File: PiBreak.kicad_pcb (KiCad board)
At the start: 2 copper layers, 56 x 62.9 mm, 318 parts, among them P1 RASPBERRY_PI_P1, P2 CONN_17, P3 CONN_8, P4 CONN_8, P5 CONN_8, P6 CONN_4X2

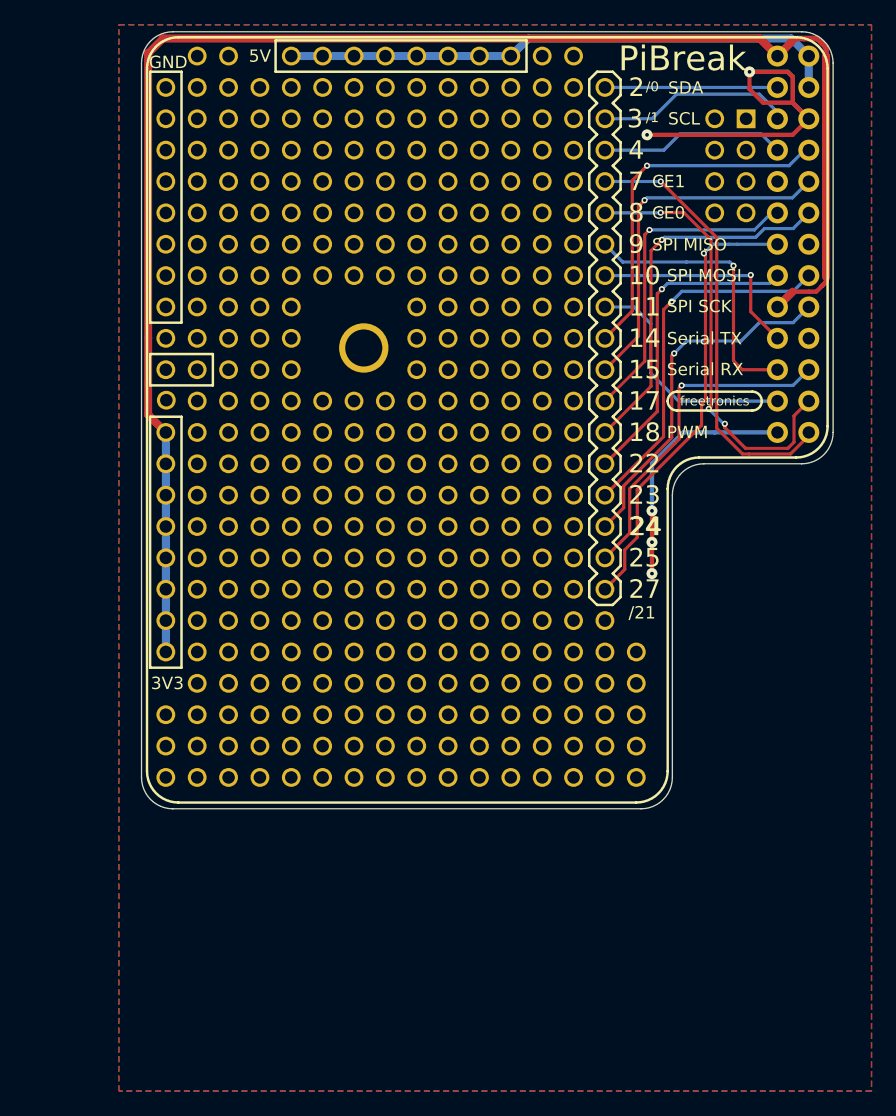
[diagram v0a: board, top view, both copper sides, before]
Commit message: Bump version to 1.0
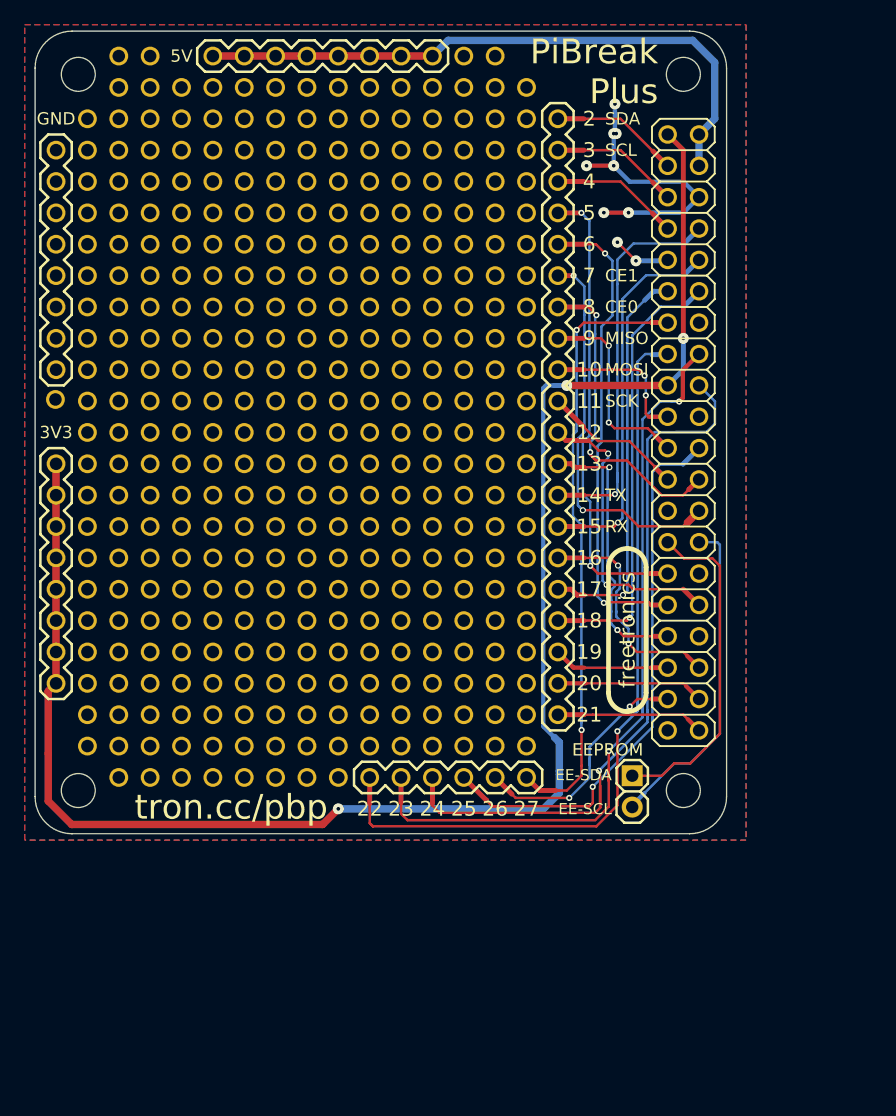
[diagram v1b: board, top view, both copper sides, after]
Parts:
- removed the 1pin_prototyping at (214.7, 124.4)
- removed the 1pin_prototyping at (224.8, 154.9)
- removed the 1pin_prototyping at (245.1, 147.3)
- removed the 1pin_prototyping at (247.7, 147.3)
- removed the 1pin_prototyping at (247.7, 142.2)
- removed the 1pin_prototyping at (245.1, 142.2)
- removed the 1pin_prototyping at (242.6, 142.2)
- removed the 1pin_prototyping at (240.0, 142.2)
- removed the 1pin_prototyping at (240.0, 144.8)
- removed the 1pin_prototyping at (242.6, 144.8)
- removed the 1pin_prototyping at (245.1, 144.8)
- removed the 1pin_prototyping at (247.7, 144.8)
- removed the 1pin_prototyping at (227.3, 154.9)
- removed the 1pin_prototyping at (227.3, 149.9)
- removed the 1pin_prototyping at (224.8, 149.9)
- removed the 1pin_prototyping at (222.2, 149.9)
- removed the 1pin_prototyping at (219.7, 149.9)
- removed the 1pin_prototyping at (219.7, 147.3)
- removed the 1pin_prototyping at (222.2, 147.3)
- removed the 1pin_prototyping at (224.8, 147.3)
- removed the 1pin_prototyping at (227.3, 147.3)
- removed the 1pin_prototyping at (227.3, 142.2)
- removed the 1pin_prototyping at (224.8, 142.2)
- removed the 1pin_prototyping at (247.7, 152.4)
- removed the 1pin_prototyping at (222.2, 142.2)
- removed the 1pin_prototyping at (219.7, 142.2)
- removed the 1pin_prototyping at (219.7, 144.8)
- removed the 1pin_prototyping at (222.2, 144.8)
- removed the 1pin_prototyping at (224.8, 144.8)
- removed the 1pin_prototyping at (227.3, 144.8)
- removed the 1pin_prototyping at (227.3, 137.2)
- removed the 1pin_prototyping at (224.8, 137.2)
- removed the 1pin_prototyping at (222.2, 137.2)
- removed the 1pin_prototyping at (219.7, 137.2)
- removed the 1pin_prototyping at (245.1, 152.4)
- removed the 1pin_prototyping at (219.7, 139.7)
- removed the 1pin_prototyping at (222.2, 139.7)
- removed the 1pin_prototyping at (224.8, 139.7)
- removed the 1pin_prototyping at (227.3, 139.7)
- removed the 1pin_prototyping at (247.7, 137.2)
- removed the 1pin_prototyping at (245.1, 137.2)
- removed the 1pin_prototyping at (242.6, 137.2)
- removed the 1pin_prototyping at (240.0, 137.2)
- removed the 1pin_prototyping at (240.0, 139.7)
- removed the 1pin_prototyping at (242.6, 139.7)
- removed the 1pin_prototyping at (242.6, 152.4)
- removed the 1pin_prototyping at (245.1, 139.7)
- removed the 1pin_prototyping at (247.7, 139.7)
- removed the 1pin_prototyping at (237.5, 139.7)
- removed the 1pin_prototyping at (234.9, 139.7)
- removed the 1pin_prototyping at (232.4, 139.7)
- removed the 1pin_prototyping at (229.9, 139.7)
- removed the 1pin_prototyping at (229.9, 137.2)
- removed the 1pin_prototyping at (232.4, 137.2)
- removed the 1pin_prototyping at (234.9, 137.2)
- removed the 1pin_prototyping at (237.5, 137.2)
- removed the 1pin_prototyping at (240.0, 152.4)
- removed the 1pin_prototyping at (237.5, 119.4)
- removed the 1pin_prototyping at (234.9, 119.4)
- removed the 1pin_prototyping at (234.9, 121.9)
- removed the 1pin_prototyping at (237.5, 121.9)
- removed the 1pin_prototyping at (247.7, 121.9)
- removed the 1pin_prototyping at (245.1, 121.9)
- removed the 1pin_prototyping at (242.6, 121.9)
- removed the 1pin_prototyping at (240.0, 121.9)
- removed the 1pin_prototyping at (240.0, 119.4)
- removed the 1pin_prototyping at (242.6, 119.4)
- removed the 1pin_prototyping at (240.0, 154.9)
- removed the 1pin_prototyping at (245.1, 119.4)
- removed the 1pin_prototyping at (247.7, 119.4)
- removed the 1pin_prototyping at (224.8, 121.9)
- removed the 1pin_prototyping at (222.2, 121.9)
- removed the 1pin_prototyping at (219.7, 121.9)
- removed the 1pin_prototyping at (219.7, 119.4)
- removed the 1pin_prototyping at (222.2, 119.4)
- removed the 1pin_prototyping at (224.8, 119.4)
- removed the 1pin_prototyping at (227.3, 127.0)
- removed the 1pin_prototyping at (224.8, 127.0)
- removed the 1pin_prototyping at (242.6, 154.9)
- removed the 1pin_prototyping at (222.2, 127.0)
- removed the 1pin_prototyping at (219.7, 127.0)
- removed the 1pin_prototyping at (219.7, 124.5)
- removed the 1pin_prototyping at (222.2, 124.5)
- removed the 1pin_prototyping at (224.8, 124.5)
- removed the 1pin_prototyping at (227.3, 124.5)
- removed the 1pin_prototyping at (227.3, 129.5)
- removed the 1pin_prototyping at (224.8, 129.5)
- removed the 1pin_prototyping at (222.2, 129.5)
- removed the 1pin_prototyping at (219.7, 129.5)
- removed the 1pin_prototyping at (245.1, 154.9)
- removed the 1pin_prototyping at (219.7, 132.1)
- removed the 1pin_prototyping at (222.2, 132.1)
- removed the 1pin_prototyping at (224.8, 132.1)
- removed the 1pin_prototyping at (227.3, 132.1)
- removed the 1pin_prototyping at (247.7, 127.0)
- removed the 1pin_prototyping at (245.1, 127.0)
- removed the 1pin_prototyping at (242.6, 127.0)
- removed the 1pin_prototyping at (240.0, 127.0)
- removed the 1pin_prototyping at (240.0, 124.5)
- removed the 1pin_prototyping at (242.6, 124.5)
- removed the 1pin_prototyping at (247.7, 154.9)
- removed the 1pin_prototyping at (245.1, 124.5)
- removed the 1pin_prototyping at (247.7, 124.5)
- removed the 1pin_prototyping at (247.7, 129.5)
- removed the 1pin_prototyping at (245.1, 129.5)
- removed the 1pin_prototyping at (242.6, 129.5)
- removed the 1pin_prototyping at (240.0, 129.5)
- removed the 1pin_prototyping at (240.0, 132.1)
- removed the 1pin_prototyping at (242.6, 132.1)
- removed the 1pin_prototyping at (245.1, 132.1)
- removed the 1pin_prototyping at (247.7, 132.1)
- removed the 1pin_prototyping at (214.6, 119.4)
- removed the 1pin_prototyping at (237.5, 154.9)
- removed the 1pin_prototyping at (237.5, 132.1)
- removed the 1pin_prototyping at (234.9, 132.1)
- removed the 1pin_prototyping at (232.4, 132.1)
- removed the 1pin_prototyping at (229.9, 132.1)
- removed the 1pin_prototyping at (229.9, 129.5)
- removed the 1pin_prototyping at (232.4, 129.5)
- removed the 1pin_prototyping at (234.9, 129.5)
- removed the 1pin_prototyping at (237.5, 129.5)
- removed the 1pin_prototyping at (237.5, 124.5)
- removed the 1pin_prototyping at (234.9, 124.5)
- removed the 1pin_prototyping at (234.9, 154.9)
- removed the 1pin_prototyping at (232.4, 124.5)
- removed the 1pin_prototyping at (229.9, 124.5)
- removed the 1pin_prototyping at (229.9, 127.0)
- removed the 1pin_prototyping at (232.4, 127.0)
- removed the 1pin_prototyping at (234.9, 127.0)
- removed the 1pin_prototyping at (237.5, 127.0)
- removed the 1pin_prototyping at (237.5, 111.8)
- removed the 1pin_prototyping at (234.9, 111.8)
- removed the 1pin_prototyping at (232.4, 111.8)
- removed the 1pin_prototyping at (229.9, 111.8)
- removed the 1pin_prototyping at (232.4, 154.9)
- removed the 1pin_prototyping at (229.9, 109.2)
- removed the 1pin_prototyping at (232.4, 109.2)
- removed the 1pin_prototyping at (234.9, 109.2)
- removed the 1pin_prototyping at (237.5, 109.2)
- removed the 1pin_prototyping at (237.5, 114.3)
- removed the 1pin_prototyping at (234.9, 114.3)
- removed the 1pin_prototyping at (232.4, 114.3)
- removed the 1pin_prototyping at (229.9, 114.3)
- removed the 1pin_prototyping at (234.9, 116.8)
- removed the 1pin_prototyping at (237.5, 116.8)
- removed the 1pin_prototyping at (229.9, 154.9)
- removed the 1pin_prototyping at (247.7, 116.8)
- removed the 1pin_prototyping at (245.1, 116.8)
- removed the 1pin_prototyping at (242.6, 116.8)
- removed the 1pin_prototyping at (240.0, 116.8)
- removed the 1pin_prototyping at (240.0, 114.3)
- removed the 1pin_prototyping at (242.6, 114.3)
- removed the 1pin_prototyping at (245.1, 114.3)
- removed the 1pin_prototyping at (247.7, 114.3)
- removed the 1pin_prototyping at (247.7, 109.2)
- removed the 1pin_prototyping at (245.1, 109.2)
- removed the 1pin_prototyping at (229.9, 152.4)
- removed the 1pin_prototyping at (242.6, 109.2)
- removed the 1pin_prototyping at (240.0, 109.2)
- removed the 1pin_prototyping at (240.0, 111.8)
- removed the 1pin_prototyping at (242.6, 111.8)
- removed the 1pin_prototyping at (245.1, 111.8)
- removed the 1pin_prototyping at (247.7, 111.8)
- removed the 1pin_prototyping at (224.8, 116.8)
- removed the 1pin_prototyping at (222.2, 116.8)
- removed the 1pin_prototyping at (219.7, 116.8)
- removed the 1pin_prototyping at (219.7, 114.3)
- removed the 1pin_prototyping at (232.4, 152.4)
- removed the 1pin_prototyping at (222.2, 114.3)
- removed the 1pin_prototyping at (224.8, 114.3)
- removed the 1pin_prototyping at (227.3, 114.3)
- removed the 1pin_prototyping at (227.3, 109.2)
- removed the 1pin_prototyping at (224.8, 109.2)
- removed the 1pin_prototyping at (222.2, 109.2)
- removed the 1pin_prototyping at (219.7, 109.2)
- removed the 1pin_prototyping at (219.7, 111.8)
- removed the 1pin_prototyping at (222.2, 111.8)
- removed the 1pin_prototyping at (224.8, 111.8)
- removed the 1pin_prototyping at (234.9, 152.4)
- removed the 1pin_prototyping at (227.3, 111.8)
- removed the 1pin_prototyping at (219.7, 96.5)
- removed the 1pin_prototyping at (227.3, 101.6)
- removed the 1pin_prototyping at (224.8, 101.6)
- removed the 1pin_prototyping at (222.2, 101.6)
- removed the 1pin_prototyping at (219.7, 101.6)
- removed the 1pin_prototyping at (219.7, 99.1)
- removed the 1pin_prototyping at (222.2, 99.1)
- removed the 1pin_prototyping at (224.8, 99.1)
- removed the 1pin_prototyping at (227.3, 99.1)
- removed the 1pin_prototyping at (237.5, 152.4)
- removed the 1pin_prototyping at (227.3, 104.1)
- removed the 1pin_prototyping at (224.8, 104.1)
- removed the 1pin_prototyping at (222.2, 104.1)
- removed the 1pin_prototyping at (219.7, 104.1)
- removed the 1pin_prototyping at (219.7, 106.7)
- removed the 1pin_prototyping at (222.2, 106.7)
- removed the 1pin_prototyping at (224.8, 106.7)
- removed the 1pin_prototyping at (227.3, 106.7)
- removed the 1pin_prototyping at (247.7, 96.5)
- removed the 1pin_prototyping at (245.1, 96.5)
- removed the 1pin_prototyping at (252.7, 154.9)
- removed the 1pin_prototyping at (247.7, 101.6)
- removed the 1pin_prototyping at (245.1, 101.6)
- removed the 1pin_prototyping at (242.6, 101.6)
- removed the 1pin_prototyping at (240.0, 101.6)
- removed the 1pin_prototyping at (240.0, 99.1)
- removed the 1pin_prototyping at (242.6, 99.1)
- removed the 1pin_prototyping at (245.1, 99.1)
- removed the 1pin_prototyping at (247.7, 99.1)
- removed the 1pin_prototyping at (247.7, 104.1)
- removed the 1pin_prototyping at (245.1, 104.1)
- removed the 1pin_prototyping at (250.2, 154.9)
- removed the 1pin_prototyping at (242.6, 104.1)
- removed the 1pin_prototyping at (240.0, 104.1)
- removed the 1pin_prototyping at (240.0, 106.7)
- removed the 1pin_prototyping at (242.6, 106.7)
- removed the 1pin_prototyping at (245.1, 106.7)
- removed the 1pin_prototyping at (247.7, 106.7)
- removed the 1pin_prototyping at (237.5, 106.7)
- removed the 1pin_prototyping at (234.9, 106.7)
- removed the 1pin_prototyping at (232.4, 106.7)
- removed the 1pin_prototyping at (229.9, 106.7)
- removed the 1pin_prototyping at (217.2, 121.9)
- removed the 1pin_prototyping at (250.2, 152.4)
- removed the 1pin_prototyping at (229.9, 104.1)
- removed the 1pin_prototyping at (232.4, 104.1)
- removed the 1pin_prototyping at (234.9, 104.1)
- removed the 1pin_prototyping at (237.5, 104.1)
- removed the 1pin_prototyping at (237.5, 99.1)
- removed the 1pin_prototyping at (234.9, 99.1)
- removed the 1pin_prototyping at (232.4, 99.1)
- removed the 1pin_prototyping at (229.9, 99.1)
- removed the 1pin_prototyping at (229.9, 101.6)
- removed the 1pin_prototyping at (232.4, 101.6)
- removed the 1pin_prototyping at (252.7, 152.4)
- removed the 1pin_prototyping at (234.9, 101.6)
- removed the 1pin_prototyping at (237.5, 101.6)
- removed the 1pin_prototyping at (217.2, 154.9)
- removed the 1pin_prototyping at (214.6, 154.9)
- removed the 1pin_prototyping at (214.6, 152.4)
- removed the 1pin_prototyping at (217.2, 152.4)
- removed the 1pin_prototyping at (217.2, 106.7)
- removed the 1pin_prototyping at (217.2, 104.1)
- removed the 1pin_prototyping at (217.2, 99.1)
- removed the 1pin_prototyping at (217.2, 101.6)
- removed the 1pin_prototyping at (227.3, 152.4)
- removed the 1pin_prototyping at (217.2, 96.5)
- removed the 1pin_prototyping at (217.2, 111.8)
- removed the 1pin_prototyping at (217.2, 109.2)
- removed the 1pin_prototyping at (217.2, 114.3)
- removed the 1pin_prototyping at (217.2, 116.8)
- removed the 1pin_prototyping at (217.2, 132.1)
- removed the 1pin_prototyping at (217.2, 129.5)
- removed the 1pin_prototyping at (217.2, 124.5)
- removed the 1pin_prototyping at (217.2, 127.0)
- removed the 1pin_prototyping at (217.2, 119.4)
- removed the 1pin_prototyping at (224.8, 152.4)
- removed the 1pin_prototyping at (214.6, 121.9)
- removed the 1pin_prototyping at (217.2, 139.7)
- removed the 1pin_prototyping at (217.2, 137.2)
- removed the 1pin_prototyping at (217.2, 134.6)
- removed the 1pin_prototyping at (217.2, 144.8)
- removed the 1pin_prototyping at (217.2, 142.2)
- removed the 1pin_prototyping at (217.2, 147.3)
- removed the 1pin_prototyping at (214.6, 149.9)
- removed the 1pin_prototyping at (217.2, 149.9)
- removed the 1pin_prototyping at (252.7, 144.8)
- removed the 1pin_prototyping at (222.2, 152.4)
- removed the 1pin_prototyping at (250.2, 144.8)
- removed the 1pin_prototyping at (250.2, 142.2)
- removed the 1pin_prototyping at (252.7, 147.3)
- removed the 1pin_prototyping at (250.2, 147.3)
- removed the 1pin_prototyping at (250.2, 149.9)
- removed the 1pin_prototyping at (252.7, 149.9)
- removed the 1pin_prototyping at (219.7, 134.6)
- removed the 1pin_prototyping at (222.2, 134.6)
- removed the 1pin_prototyping at (224.8, 134.6)
- removed the 1pin_prototyping at (227.3, 134.6)
- removed the 1pin_prototyping at (219.7, 152.4)
- removed the 1pin_prototyping at (240.0, 134.6)
- removed the 1pin_prototyping at (242.6, 134.6)
- removed the 1pin_prototyping at (245.1, 134.6)
- removed the 1pin_prototyping at (247.7, 134.6)
- removed the 1pin_prototyping at (237.5, 134.6)
- removed the 1pin_prototyping at (234.9, 134.6)
- removed the 1pin_prototyping at (232.4, 134.6)
- removed the 1pin_prototyping at (229.9, 134.6)
- removed the 1pin_prototyping at (237.5, 144.8)
- removed the 1pin_prototyping at (234.9, 144.8)
- removed the 1pin_prototyping at (219.7, 154.9)
- removed the 1pin_prototyping at (232.4, 144.8)
- removed the 1pin_prototyping at (229.9, 144.8)
- removed the 1pin_prototyping at (229.9, 142.2)
- removed the 1pin_prototyping at (232.4, 142.2)
- removed the 1pin_prototyping at (234.9, 142.2)
- removed the 1pin_prototyping at (237.5, 142.2)
- removed the 1pin_prototyping at (237.5, 147.3)
- removed the 1pin_prototyping at (234.9, 147.3)
- removed the 1pin_prototyping at (232.4, 147.3)
- removed the 1pin_prototyping at (229.9, 147.3)
- removed the 1pin_prototyping at (222.2, 154.9)
- removed the 1pin_prototyping at (229.9, 149.9)
- removed the 1pin_prototyping at (232.4, 149.9)
- removed the 1pin_prototyping at (234.9, 149.9)
- removed the 1pin_prototyping at (237.5, 149.9)
- removed the 1pin_prototyping at (247.7, 149.9)
- removed the 1pin_prototyping at (245.1, 149.9)
- removed the 1pin_prototyping at (242.6, 149.9)
- removed the 1pin_prototyping at (240.0, 149.9)
- removed the 1pin_prototyping at (240.0, 147.3)
- removed the 1pin_prototyping at (242.6, 147.3)
- removed LOGO_FREETRONICS_SMALL: val**, LOGO_FREETRONICS_SMALL
- added 1PIN: P***, Connect:1pin, F.Cu at (256.8, 99.0)
- added 1PIN: P***, Connect:1pin, F.Cu at (248.8, 98.0)
- added 1PIN: P***, Connect:1pin, F.Cu at (250.2, 156.2)
- added 1PIN: P***, Connect:1pin, F.Cu at (256.8, 157.0)
- added 1pin_prototyping: val**, FT:1pin_prototyping, F.Cu at (210.8, 96.5)
- added 1pin_prototyping: val**, FT:1pin_prototyping, F.Cu at (208.3, 106.7)
- added 1pin_prototyping: val**, FT:1pin_prototyping, F.Cu at (210.8, 106.7)
- added 1pin_prototyping: val**, FT:1pin_prototyping, F.Cu at (210.8, 101.6)
- added 1pin_prototyping: val**, FT:1pin_prototyping, F.Cu at (213.4, 101.6)
- added 1pin_prototyping: val**, FT:1pin_prototyping, F.Cu at (213.4, 104.1)
- added 1pin_prototyping: val**, FT:1pin_prototyping, F.Cu at (210.8, 104.1)
- added 1pin_prototyping: val**, FT:1pin_prototyping, F.Cu at (213.4, 111.8)
- added 1pin_prototyping: val**, FT:1pin_prototyping, F.Cu at (210.8, 111.8)
- added 1pin_prototyping: val**, FT:1pin_prototyping, F.Cu at (215.9, 111.8)
- added 1pin_prototyping: val**, FT:1pin_prototyping, F.Cu at (218.4, 111.8)
- added 1pin_prototyping: val**, FT:1pin_prototyping, F.Cu at (221.0, 111.8)
- added 1pin_prototyping: val**, FT:1pin_prototyping, F.Cu at (208.3, 109.2)
- added 1pin_prototyping: val**, FT:1pin_prototyping, F.Cu at (223.5, 111.8)
- added 1pin_prototyping: val**, FT:1pin_prototyping, F.Cu at (226.1, 111.8)
- added 1pin_prototyping: val**, FT:1pin_prototyping, F.Cu at (228.6, 111.8)
- added 1pin_prototyping: val**, FT:1pin_prototyping, F.Cu at (243.8, 111.8)
- added 1pin_prototyping: val**, FT:1pin_prototyping, F.Cu at (241.3, 111.8)
- added 1pin_prototyping: val**, FT:1pin_prototyping, F.Cu at (238.8, 111.8)
- added 1pin_prototyping: val**, FT:1pin_prototyping, F.Cu at (236.2, 111.8)
- added 1pin_prototyping: val**, FT:1pin_prototyping, F.Cu at (233.7, 111.8)
- added 1pin_prototyping: val**, FT:1pin_prototyping, F.Cu at (231.1, 111.8)
- added 1pin_prototyping: val**, FT:1pin_prototyping, F.Cu at (231.1, 132.1)
- added 1pin_prototyping: val**, FT:1pin_prototyping, F.Cu at (208.3, 124.5)
- added 1pin_prototyping: val**, FT:1pin_prototyping, F.Cu at (233.7, 132.1)
- added 1pin_prototyping: val**, FT:1pin_prototyping, F.Cu at (236.2, 132.1)
- added 1pin_prototyping: val**, FT:1pin_prototyping, F.Cu at (238.8, 132.1)
- added 1pin_prototyping: val**, FT:1pin_prototyping, F.Cu at (241.3, 132.1)
- added 1pin_prototyping: val**, FT:1pin_prototyping, F.Cu at (241.3, 129.5)
- added 1pin_prototyping: val**, FT:1pin_prototyping, F.Cu at (238.8, 129.5)
- added 1pin_prototyping: val**, FT:1pin_prototyping, F.Cu at (236.2, 129.5)
- added 1pin_prototyping: val**, FT:1pin_prototyping, F.Cu at (233.7, 129.5)
- added 1pin_prototyping: val**, FT:1pin_prototyping, F.Cu at (231.1, 129.5)
- added 1pin_prototyping: val**, FT:1pin_prototyping, F.Cu at (231.1, 124.5)
- added 1pin_prototyping: val**, FT:1pin_prototyping, F.Cu at (205.7, 124.3)
- added 1pin_prototyping: val**, FT:1pin_prototyping, F.Cu at (233.7, 124.5)
- added 1pin_prototyping: val**, FT:1pin_prototyping, F.Cu at (236.2, 124.5)
- added 1pin_prototyping: val**, FT:1pin_prototyping, F.Cu at (238.8, 124.5)
- added 1pin_prototyping: val**, FT:1pin_prototyping, F.Cu at (241.3, 124.5)
- added 1pin_prototyping: val**, FT:1pin_prototyping, F.Cu at (241.3, 127.0)
- added 1pin_prototyping: val**, FT:1pin_prototyping, F.Cu at (238.8, 127.0)
- added 1pin_prototyping: val**, FT:1pin_prototyping, F.Cu at (236.2, 127.0)
- added 1pin_prototyping: val**, FT:1pin_prototyping, F.Cu at (233.7, 127.0)
- added 1pin_prototyping: val**, FT:1pin_prototyping, F.Cu at (231.1, 127.0)
- added 1pin_prototyping: val**, FT:1pin_prototyping, F.Cu at (243.8, 127.0)
- added 1pin_prototyping: val**, FT:1pin_prototyping, F.Cu at (228.6, 154.9)
- added 1pin_prototyping: val**, FT:1pin_prototyping, F.Cu at (243.8, 124.5)
- added 1pin_prototyping: val**, FT:1pin_prototyping, F.Cu at (243.8, 129.5)
- added 1pin_prototyping: val**, FT:1pin_prototyping, F.Cu at (243.8, 132.1)
- added 1pin_prototyping: val**, FT:1pin_prototyping, F.Cu at (228.6, 132.1)
- added 1pin_prototyping: val**, FT:1pin_prototyping, F.Cu at (228.6, 129.5)
- added 1pin_prototyping: val**, FT:1pin_prototyping, F.Cu at (228.6, 124.5)
- added 1pin_prototyping: val**, FT:1pin_prototyping, F.Cu at (228.6, 127.0)
- added 1pin_prototyping: val**, FT:1pin_prototyping, F.Cu at (215.9, 127.0)
- added 1pin_prototyping: val**, FT:1pin_prototyping, F.Cu at (218.4, 127.0)
- added 1pin_prototyping: val**, FT:1pin_prototyping, F.Cu at (221.0, 127.0)
- added 1pin_prototyping: val**, FT:1pin_prototyping, F.Cu at (226.1, 154.9)
- added 1pin_prototyping: val**, FT:1pin_prototyping, F.Cu at (223.5, 127.0)
- added 1pin_prototyping: val**, FT:1pin_prototyping, F.Cu at (226.1, 127.0)
- added 1pin_prototyping: val**, FT:1pin_prototyping, F.Cu at (226.1, 124.5)
- added 1pin_prototyping: val**, FT:1pin_prototyping, F.Cu at (223.5, 124.5)
- added 1pin_prototyping: val**, FT:1pin_prototyping, F.Cu at (221.0, 124.5)
- added 1pin_prototyping: val**, FT:1pin_prototyping, F.Cu at (218.4, 124.5)
- added 1pin_prototyping: val**, FT:1pin_prototyping, F.Cu at (215.9, 124.5)
- added 1pin_prototyping: val**, FT:1pin_prototyping, F.Cu at (215.9, 129.5)
- added 1pin_prototyping: val**, FT:1pin_prototyping, F.Cu at (218.4, 129.5)
- added 1pin_prototyping: val**, FT:1pin_prototyping, F.Cu at (221.0, 129.5)
- added 1pin_prototyping: val**, FT:1pin_prototyping, F.Cu at (223.5, 154.9)
- added 1pin_prototyping: val**, FT:1pin_prototyping, F.Cu at (223.5, 129.5)
- added 1pin_prototyping: val**, FT:1pin_prototyping, F.Cu at (226.1, 129.5)
- added 1pin_prototyping: val**, FT:1pin_prototyping, F.Cu at (226.1, 132.1)
- added 1pin_prototyping: val**, FT:1pin_prototyping, F.Cu at (223.5, 132.1)
- added 1pin_prototyping: val**, FT:1pin_prototyping, F.Cu at (221.0, 132.1)
- added 1pin_prototyping: val**, FT:1pin_prototyping, F.Cu at (218.4, 132.1)
- added 1pin_prototyping: val**, FT:1pin_prototyping, F.Cu at (215.9, 132.1)
- added 1pin_prototyping: val**, FT:1pin_prototyping, F.Cu at (210.8, 132.1)
- added 1pin_prototyping: val**, FT:1pin_prototyping, F.Cu at (213.4, 132.1)
- added 1pin_prototyping: val**, FT:1pin_prototyping, F.Cu at (213.4, 129.5)
- added 1pin_prototyping: val**, FT:1pin_prototyping, F.Cu at (221.0, 154.9)
- added 1pin_prototyping: val**, FT:1pin_prototyping, F.Cu at (210.8, 129.5)
- added 1pin_prototyping: val**, FT:1pin_prototyping, F.Cu at (210.8, 124.5)
- added 1pin_prototyping: val**, FT:1pin_prototyping, F.Cu at (213.4, 124.5)
- added 1pin_prototyping: val**, FT:1pin_prototyping, F.Cu at (213.4, 127.0)
- added 1pin_prototyping: val**, FT:1pin_prototyping, F.Cu at (210.8, 127.0)
- added 1pin_prototyping: val**, FT:1pin_prototyping, F.Cu at (210.8, 116.8)
- added 1pin_prototyping: val**, FT:1pin_prototyping, F.Cu at (213.4, 116.8)
- added 1pin_prototyping: val**, FT:1pin_prototyping, F.Cu at (213.4, 114.3)
- added 1pin_prototyping: val**, FT:1pin_prototyping, F.Cu at (210.8, 114.3)
- added 1pin_prototyping: val**, FT:1pin_prototyping, F.Cu at (210.8, 119.4)
- added 1pin_prototyping: val**, FT:1pin_prototyping, F.Cu at (218.4, 154.9)
- added 1pin_prototyping: val**, FT:1pin_prototyping, F.Cu at (213.4, 119.4)
- added 1pin_prototyping: val**, FT:1pin_prototyping, F.Cu at (213.4, 121.9)
- added 1pin_prototyping: val**, FT:1pin_prototyping, F.Cu at (210.8, 121.9)
- added 1pin_prototyping: val**, FT:1pin_prototyping, F.Cu at (215.9, 121.9)
- added 1pin_prototyping: val**, FT:1pin_prototyping, F.Cu at (218.4, 121.9)
- added 1pin_prototyping: val**, FT:1pin_prototyping, F.Cu at (221.0, 121.9)
- added 1pin_prototyping: val**, FT:1pin_prototyping, F.Cu at (223.5, 121.9)
- added 1pin_prototyping: val**, FT:1pin_prototyping, F.Cu at (226.1, 121.9)
- added 1pin_prototyping: val**, FT:1pin_prototyping, F.Cu at (226.1, 119.4)
- added 1pin_prototyping: val**, FT:1pin_prototyping, F.Cu at (223.5, 119.4)
- added 1pin_prototyping: val**, FT:1pin_prototyping, F.Cu at (215.9, 154.9)
- added 1pin_prototyping: val**, FT:1pin_prototyping, F.Cu at (221.0, 119.4)
- added 1pin_prototyping: val**, FT:1pin_prototyping, F.Cu at (218.4, 119.4)
- added 1pin_prototyping: val**, FT:1pin_prototyping, F.Cu at (215.9, 119.4)
- added 1pin_prototyping: val**, FT:1pin_prototyping, F.Cu at (215.9, 114.3)
- added 1pin_prototyping: val**, FT:1pin_prototyping, F.Cu at (218.4, 114.3)
- added 1pin_prototyping: val**, FT:1pin_prototyping, F.Cu at (221.0, 114.3)
- added 1pin_prototyping: val**, FT:1pin_prototyping, F.Cu at (223.5, 114.3)
- added 1pin_prototyping: val**, FT:1pin_prototyping, F.Cu at (226.1, 114.3)
- added 1pin_prototyping: val**, FT:1pin_prototyping, F.Cu at (226.1, 116.8)
- added 1pin_prototyping: val**, FT:1pin_prototyping, F.Cu at (223.5, 116.8)
- added 1pin_prototyping: val**, FT:1pin_prototyping, F.Cu at (213.4, 96.5)
- added 1pin_prototyping: val**, FT:1pin_prototyping, F.Cu at (210.8, 154.9)
- added 1pin_prototyping: val**, FT:1pin_prototyping, F.Cu at (221.0, 116.8)
- added 1pin_prototyping: val**, FT:1pin_prototyping, F.Cu at (218.4, 116.8)
- added 1pin_prototyping: val**, FT:1pin_prototyping, F.Cu at (215.9, 116.8)
- added 1pin_prototyping: val**, FT:1pin_prototyping, F.Cu at (228.6, 116.8)
- added 1pin_prototyping: val**, FT:1pin_prototyping, F.Cu at (228.6, 114.3)
- added 1pin_prototyping: val**, FT:1pin_prototyping, F.Cu at (228.6, 119.4)
- added 1pin_prototyping: val**, FT:1pin_prototyping, F.Cu at (228.6, 121.9)
- added 1pin_prototyping: val**, FT:1pin_prototyping, F.Cu at (243.8, 121.9)
- added 1pin_prototyping: val**, FT:1pin_prototyping, F.Cu at (243.8, 119.4)
- added 1pin_prototyping: val**, FT:1pin_prototyping, F.Cu at (243.8, 114.3)
- added 1pin_prototyping: val**, FT:1pin_prototyping, F.Cu at (213.4, 154.9)
- added 1pin_prototyping: val**, FT:1pin_prototyping, F.Cu at (243.8, 116.8)
- added 1pin_prototyping: val**, FT:1pin_prototyping, F.Cu at (231.1, 116.8)
- added 1pin_prototyping: val**, FT:1pin_prototyping, F.Cu at (233.7, 116.8)
- added 1pin_prototyping: val**, FT:1pin_prototyping, F.Cu at (236.2, 116.8)
- added 1pin_prototyping: val**, FT:1pin_prototyping, F.Cu at (238.8, 116.8)
- added 1pin_prototyping: val**, FT:1pin_prototyping, F.Cu at (241.3, 116.8)
- added 1pin_prototyping: val**, FT:1pin_prototyping, F.Cu at (241.3, 114.3)
- added 1pin_prototyping: val**, FT:1pin_prototyping, F.Cu at (238.8, 114.3)
- added 1pin_prototyping: val**, FT:1pin_prototyping, F.Cu at (236.2, 114.3)
- added 1pin_prototyping: val**, FT:1pin_prototyping, F.Cu at (233.7, 114.3)
- added 1pin_prototyping: val**, FT:1pin_prototyping, F.Cu at (208.3, 152.4)
- added 1pin_prototyping: val**, FT:1pin_prototyping, F.Cu at (231.1, 114.3)
- added 1pin_prototyping: val**, FT:1pin_prototyping, F.Cu at (231.1, 119.4)
- added 1pin_prototyping: val**, FT:1pin_prototyping, F.Cu at (233.7, 119.4)
- added 1pin_prototyping: val**, FT:1pin_prototyping, F.Cu at (236.2, 119.4)
- added 1pin_prototyping: val**, FT:1pin_prototyping, F.Cu at (238.8, 119.4)
- added 1pin_prototyping: val**, FT:1pin_prototyping, F.Cu at (241.3, 119.4)
- added 1pin_prototyping: val**, FT:1pin_prototyping, F.Cu at (241.3, 121.9)
- added 1pin_prototyping: val**, FT:1pin_prototyping, F.Cu at (238.8, 121.9)
- added 1pin_prototyping: val**, FT:1pin_prototyping, F.Cu at (236.2, 121.9)
- added 1pin_prototyping: val**, FT:1pin_prototyping, F.Cu at (233.7, 121.9)
- added 1pin_prototyping: val**, FT:1pin_prototyping, F.Cu at (208.3, 149.9)
- added 1pin_prototyping: val**, FT:1pin_prototyping, F.Cu at (231.1, 121.9)
- added 1pin_prototyping: val**, FT:1pin_prototyping, F.Cu at (231.1, 142.2)
- added 1pin_prototyping: val**, FT:1pin_prototyping, F.Cu at (233.7, 142.2)
- added 1pin_prototyping: val**, FT:1pin_prototyping, F.Cu at (236.2, 142.2)
- added 1pin_prototyping: val**, FT:1pin_prototyping, F.Cu at (238.8, 142.2)
- added 1pin_prototyping: val**, FT:1pin_prototyping, F.Cu at (241.3, 142.2)
- added 1pin_prototyping: val**, FT:1pin_prototyping, F.Cu at (241.3, 139.7)
- added 1pin_prototyping: val**, FT:1pin_prototyping, F.Cu at (238.8, 139.7)
- added 1pin_prototyping: val**, FT:1pin_prototyping, F.Cu at (236.2, 139.7)
- added 1pin_prototyping: val**, FT:1pin_prototyping, F.Cu at (233.7, 139.7)
- added 1pin_prototyping: val**, FT:1pin_prototyping, F.Cu at (208.3, 144.8)
- added 1pin_prototyping: val**, FT:1pin_prototyping, F.Cu at (231.1, 139.7)
- added 1pin_prototyping: val**, FT:1pin_prototyping, F.Cu at (231.1, 134.6)
- added 1pin_prototyping: val**, FT:1pin_prototyping, F.Cu at (233.7, 134.6)
- added 1pin_prototyping: val**, FT:1pin_prototyping, F.Cu at (236.2, 134.6)
- added 1pin_prototyping: val**, FT:1pin_prototyping, F.Cu at (238.8, 134.6)
- added 1pin_prototyping: val**, FT:1pin_prototyping, F.Cu at (241.3, 134.6)
- added 1pin_prototyping: val**, FT:1pin_prototyping, F.Cu at (241.3, 137.2)
- added 1pin_prototyping: val**, FT:1pin_prototyping, F.Cu at (238.8, 137.2)
- added 1pin_prototyping: val**, FT:1pin_prototyping, F.Cu at (236.2, 137.2)
- added 1pin_prototyping: val**, FT:1pin_prototyping, F.Cu at (233.7, 137.2)
- added 1pin_prototyping: val**, FT:1pin_prototyping, F.Cu at (208.3, 147.3)
- added 1pin_prototyping: val**, FT:1pin_prototyping, F.Cu at (231.1, 137.2)
- added 1pin_prototyping: val**, FT:1pin_prototyping, F.Cu at (243.8, 137.2)
- added 1pin_prototyping: val**, FT:1pin_prototyping, F.Cu at (243.8, 134.6)
- added 1pin_prototyping: val**, FT:1pin_prototyping, F.Cu at (243.8, 139.7)
- added 1pin_prototyping: val**, FT:1pin_prototyping, F.Cu at (243.8, 142.2)
- added 1pin_prototyping: val**, FT:1pin_prototyping, F.Cu at (228.6, 142.2)
- added 1pin_prototyping: val**, FT:1pin_prototyping, F.Cu at (228.6, 139.7)
- added 1pin_prototyping: val**, FT:1pin_prototyping, F.Cu at (228.6, 134.6)
- added 1pin_prototyping: val**, FT:1pin_prototyping, F.Cu at (228.6, 137.2)
- added 1pin_prototyping: val**, FT:1pin_prototyping, F.Cu at (215.9, 137.2)
- added 1pin_prototyping: val**, FT:1pin_prototyping, F.Cu at (208.3, 137.2)
- added 1pin_prototyping: val**, FT:1pin_prototyping, F.Cu at (218.4, 137.2)
- added 1pin_prototyping: val**, FT:1pin_prototyping, F.Cu at (221.0, 137.2)
- added 1pin_prototyping: val**, FT:1pin_prototyping, F.Cu at (223.5, 137.2)
- added 1pin_prototyping: val**, FT:1pin_prototyping, F.Cu at (226.1, 137.2)
- added 1pin_prototyping: val**, FT:1pin_prototyping, F.Cu at (226.1, 134.6)
- added 1pin_prototyping: val**, FT:1pin_prototyping, F.Cu at (223.5, 134.6)
- added 1pin_prototyping: val**, FT:1pin_prototyping, F.Cu at (221.0, 134.6)
- added 1pin_prototyping: val**, FT:1pin_prototyping, F.Cu at (218.4, 134.6)
- added 1pin_prototyping: val**, FT:1pin_prototyping, F.Cu at (215.9, 134.6)
- added 1pin_prototyping: val**, FT:1pin_prototyping, F.Cu at (215.9, 139.7)
- added 1pin_prototyping: val**, FT:1pin_prototyping, F.Cu at (208.3, 134.6)
- added 1pin_prototyping: val**, FT:1pin_prototyping, F.Cu at (218.4, 139.7)
- added 1pin_prototyping: val**, FT:1pin_prototyping, F.Cu at (221.0, 139.7)
- added 1pin_prototyping: val**, FT:1pin_prototyping, F.Cu at (223.5, 139.7)
- added 1pin_prototyping: val**, FT:1pin_prototyping, F.Cu at (226.1, 139.7)
- added 1pin_prototyping: val**, FT:1pin_prototyping, F.Cu at (226.1, 142.2)
- added 1pin_prototyping: val**, FT:1pin_prototyping, F.Cu at (223.5, 142.2)
- added 1pin_prototyping: val**, FT:1pin_prototyping, F.Cu at (221.0, 142.2)
- added 1pin_prototyping: val**, FT:1pin_prototyping, F.Cu at (218.4, 142.2)
- added 1pin_prototyping: val**, FT:1pin_prototyping, F.Cu at (215.9, 142.2)
- added 1pin_prototyping: val**, FT:1pin_prototyping, F.Cu at (210.8, 142.2)
- added 1pin_prototyping: val**, FT:1pin_prototyping, F.Cu at (208.3, 139.7)
- added 1pin_prototyping: val**, FT:1pin_prototyping, F.Cu at (213.4, 142.2)
- added 1pin_prototyping: val**, FT:1pin_prototyping, F.Cu at (213.4, 139.7)
- added 1pin_prototyping: val**, FT:1pin_prototyping, F.Cu at (210.8, 139.7)
- added 1pin_prototyping: val**, FT:1pin_prototyping, F.Cu at (210.8, 134.6)
- added 1pin_prototyping: val**, FT:1pin_prototyping, F.Cu at (213.4, 134.6)
- added 1pin_prototyping: val**, FT:1pin_prototyping, F.Cu at (213.4, 137.2)
- added 1pin_prototyping: val**, FT:1pin_prototyping, F.Cu at (210.8, 137.2)
- added 1pin_prototyping: val**, FT:1pin_prototyping, F.Cu at (210.8, 147.3)
- added 1pin_prototyping: val**, FT:1pin_prototyping, F.Cu at (213.4, 147.3)
- added 1pin_prototyping: val**, FT:1pin_prototyping, F.Cu at (213.4, 144.8)
- added 1pin_prototyping: val**, FT:1pin_prototyping, F.Cu at (208.3, 142.2)
- added 1pin_prototyping: val**, FT:1pin_prototyping, F.Cu at (210.8, 144.8)
- added 1pin_prototyping: val**, FT:1pin_prototyping, F.Cu at (210.8, 149.9)
- added 1pin_prototyping: val**, FT:1pin_prototyping, F.Cu at (213.4, 149.9)
- added 1pin_prototyping: val**, FT:1pin_prototyping, F.Cu at (213.4, 152.4)
- added 1pin_prototyping: val**, FT:1pin_prototyping, F.Cu at (210.8, 152.4)
- added 1pin_prototyping: val**, FT:1pin_prototyping, F.Cu at (215.9, 152.4)
- added 1pin_prototyping: val**, FT:1pin_prototyping, F.Cu at (218.4, 152.4)
- added 1pin_prototyping: val**, FT:1pin_prototyping, F.Cu at (221.0, 152.4)
- added 1pin_prototyping: val**, FT:1pin_prototyping, F.Cu at (223.5, 152.4)
- added 1pin_prototyping: val**, FT:1pin_prototyping, F.Cu at (226.1, 152.4)
- added 1pin_prototyping: val**, FT:1pin_prototyping, F.Cu at (208.3, 121.9)
- added 1pin_prototyping: val**, FT:1pin_prototyping, F.Cu at (208.3, 132.1)
- added 1pin_prototyping: val**, FT:1pin_prototyping, F.Cu at (226.1, 149.9)
- added 1pin_prototyping: val**, FT:1pin_prototyping, F.Cu at (223.5, 149.9)
- added 1pin_prototyping: val**, FT:1pin_prototyping, F.Cu at (221.0, 149.9)
- added 1pin_prototyping: val**, FT:1pin_prototyping, F.Cu at (218.4, 149.9)
- added 1pin_prototyping: val**, FT:1pin_prototyping, F.Cu at (215.9, 149.9)
- added 1pin_prototyping: val**, FT:1pin_prototyping, F.Cu at (215.9, 144.8)
- added 1pin_prototyping: val**, FT:1pin_prototyping, F.Cu at (218.4, 144.8)
- added 1pin_prototyping: val**, FT:1pin_prototyping, F.Cu at (221.0, 144.8)
- added 1pin_prototyping: val**, FT:1pin_prototyping, F.Cu at (223.5, 144.8)
- added 1pin_prototyping: val**, FT:1pin_prototyping, F.Cu at (226.1, 144.8)
- added 1pin_prototyping: val**, FT:1pin_prototyping, F.Cu at (208.3, 127.0)
- added 1pin_prototyping: val**, FT:1pin_prototyping, F.Cu at (226.1, 147.3)
- added 1pin_prototyping: val**, FT:1pin_prototyping, F.Cu at (223.5, 147.3)
- added 1pin_prototyping: val**, FT:1pin_prototyping, F.Cu at (221.0, 147.3)
- added 1pin_prototyping: val**, FT:1pin_prototyping, F.Cu at (218.4, 147.3)
- added 1pin_prototyping: val**, FT:1pin_prototyping, F.Cu at (215.9, 147.3)
- added 1pin_prototyping: val**, FT:1pin_prototyping, F.Cu at (228.6, 147.3)
- added 1pin_prototyping: val**, FT:1pin_prototyping, F.Cu at (228.6, 144.8)
- added 1pin_prototyping: val**, FT:1pin_prototyping, F.Cu at (228.6, 149.9)
- added 1pin_prototyping: val**, FT:1pin_prototyping, F.Cu at (228.6, 152.4)
- added 1pin_prototyping: val**, FT:1pin_prototyping, F.Cu at (243.8, 152.4)
- added 1pin_prototyping: val**, FT:1pin_prototyping, F.Cu at (208.3, 129.5)
- added 1pin_prototyping: val**, FT:1pin_prototyping, F.Cu at (243.8, 149.9)
- added 1pin_prototyping: val**, FT:1pin_prototyping, F.Cu at (243.8, 144.8)
- added 1pin_prototyping: val**, FT:1pin_prototyping, F.Cu at (243.8, 147.3)
- added 1pin_prototyping: val**, FT:1pin_prototyping, F.Cu at (231.1, 147.3)
- added 1pin_prototyping: val**, FT:1pin_prototyping, F.Cu at (233.7, 147.3)
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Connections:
- P2 pad 10: /GPIO15_RXD -> /GPIO11_SCK
- P2 pad 11: /GPIO17 -> /GPIO12
- P2 pad 12: /GPIO18_PCM_CLK -> /GPIO13
- P2 pad 13: /GPIO22 -> /GPIO14_TXD
- P2 pad 14: /GPIO23 -> /GPIO15_RXD
- P2 pad 15: /GPIO24 -> /GPIO16
- P2 pad 16: /GPIO25 -> /GPIO17
- P2 pad 17: /GPIO27 -> /GPIO18_PCM_CLK
- P2 pad 4: /GPIO7_CE1 -> /GPIO5
- P2 pad 5: /GPIO8_CE0 -> /GPIO6
- P2 pad 6: /GPIO9_MISO -> /GPIO7_CE1
- P2 pad 7: /GPIO10_MOSI -> /GPIO8_CE0
- P2 pad 8: /GPIO11_SCK -> /GPIO9_MISO
- P2 pad 9: /GPIO14_TXD -> /GPIO10_MOSI
- P3 pad 1: +5V -> /GPIO22
- P3 pad 2: +5V -> /GPIO23
- P3 pad 3: +5V -> /GPIO24
- P3 pad 4: +5V -> /GPIO25
- P3 pad 5: +5V -> /GPIO26
- P3 pad 6: +5V -> /GPIO27
- P4 pad 1: +3.3V -> +5V
- P4 pad 2: +3.3V -> +5V
- P4 pad 3: +3.3V -> +5V
- P4 pad 4: +3.3V -> +5V
- P4 pad 5: +3.3V -> +5V
- P4 pad 6: +3.3V -> +5V
- P4 pad 7: +3.3V -> +5V
- P4 pad 8: +3.3V -> +5V
- P5 pad 1: GND -> +3.3V
- P5 pad 2: GND -> +3.3V
- P5 pad 3: GND -> +3.3V
- P5 pad 4: GND -> +3.3V
- P5 pad 5: GND -> +3.3V
- P5 pad 6: GND -> +3.3V
- P5 pad 7: GND -> +3.3V
- P5 pad 8: GND -> +3.3V
- P6 pad 1: (no net) -> GND
- P6 pad 2: (no net) -> GND
- P6 pad 3: (no net) -> GND
- P6 pad 4: (no net) -> GND
- P6 pad 5: (no net) -> GND
- P6 pad 6: (no net) -> GND
- P6 pad 7: (no net) -> GND
- P6 pad 8: (no net) -> GND
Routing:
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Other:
- board size 56 x 62.9 mm -> 56 x 65 mm
- net class Default: trace_width 0.254 -> 0.2
- board text added: "12"
- board text added: "13"
- board text added: "16"
- board text added: "19"
- board text added: "20"
- board text added: "21"
- board text added: "26"
- board text added: "5"
- board text added: "6"
- board text added: "Copyright 2014 Freetronics Pty Ltd TAPR Open Hardware License"
- board text added: "EE-SCL"
- board text added: "EE-SDA"
- board text added: "EEPROM"
- board text added: "MISO"
- board text added: "MOSI"
- board text added: "PiBreak Plus"
- board text added: "RX"
- board text added: "SCK"
- board text added: "TX"
- board text added: "tron.cc/pbp"
- board text added: "tron.cc/pbp SKU: PIBP V1.0"
- board text removed: "/0"
- board text removed: "/1"
- board text removed: "/21"
- board text removed: "1"
- board text removed: "Copyright 2013 Freetronics Pty Ltd. TAPR Open Hardware License"
- board text removed: "PWM"
- board text removed: "PiBreak"
- board text removed: "SPI MISO"
- board text removed: "SPI MOSI"
- board text removed: "SPI SCK"
- board text removed: "Serial RX"
- board text removed: "Serial TX"
- board text removed: "V1.1 SKU: PIBR"
- board text removed: "tron.cc/pibr"
